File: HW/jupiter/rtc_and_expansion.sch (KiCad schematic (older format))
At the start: 3 parts, among them J2 Expansion Bus, U3 DS1511Y+

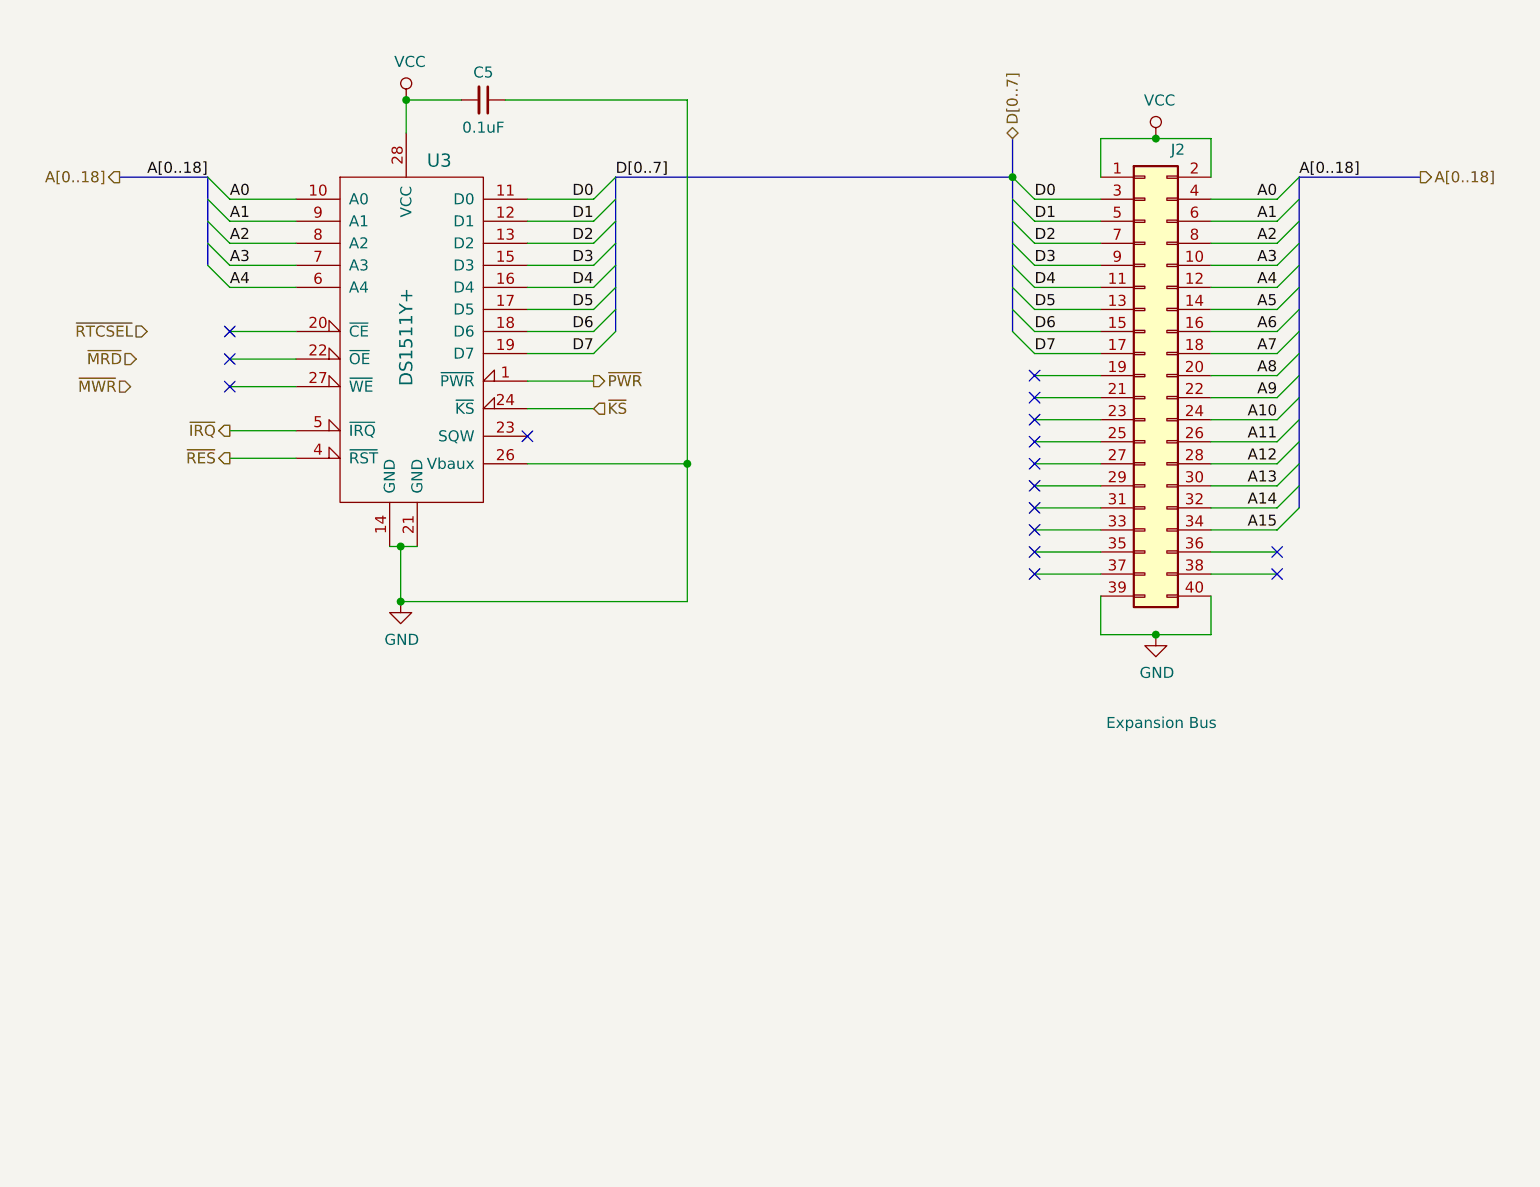
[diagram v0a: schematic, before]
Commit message: A lot of new data sheets. Some updates to schema and PCB layout.
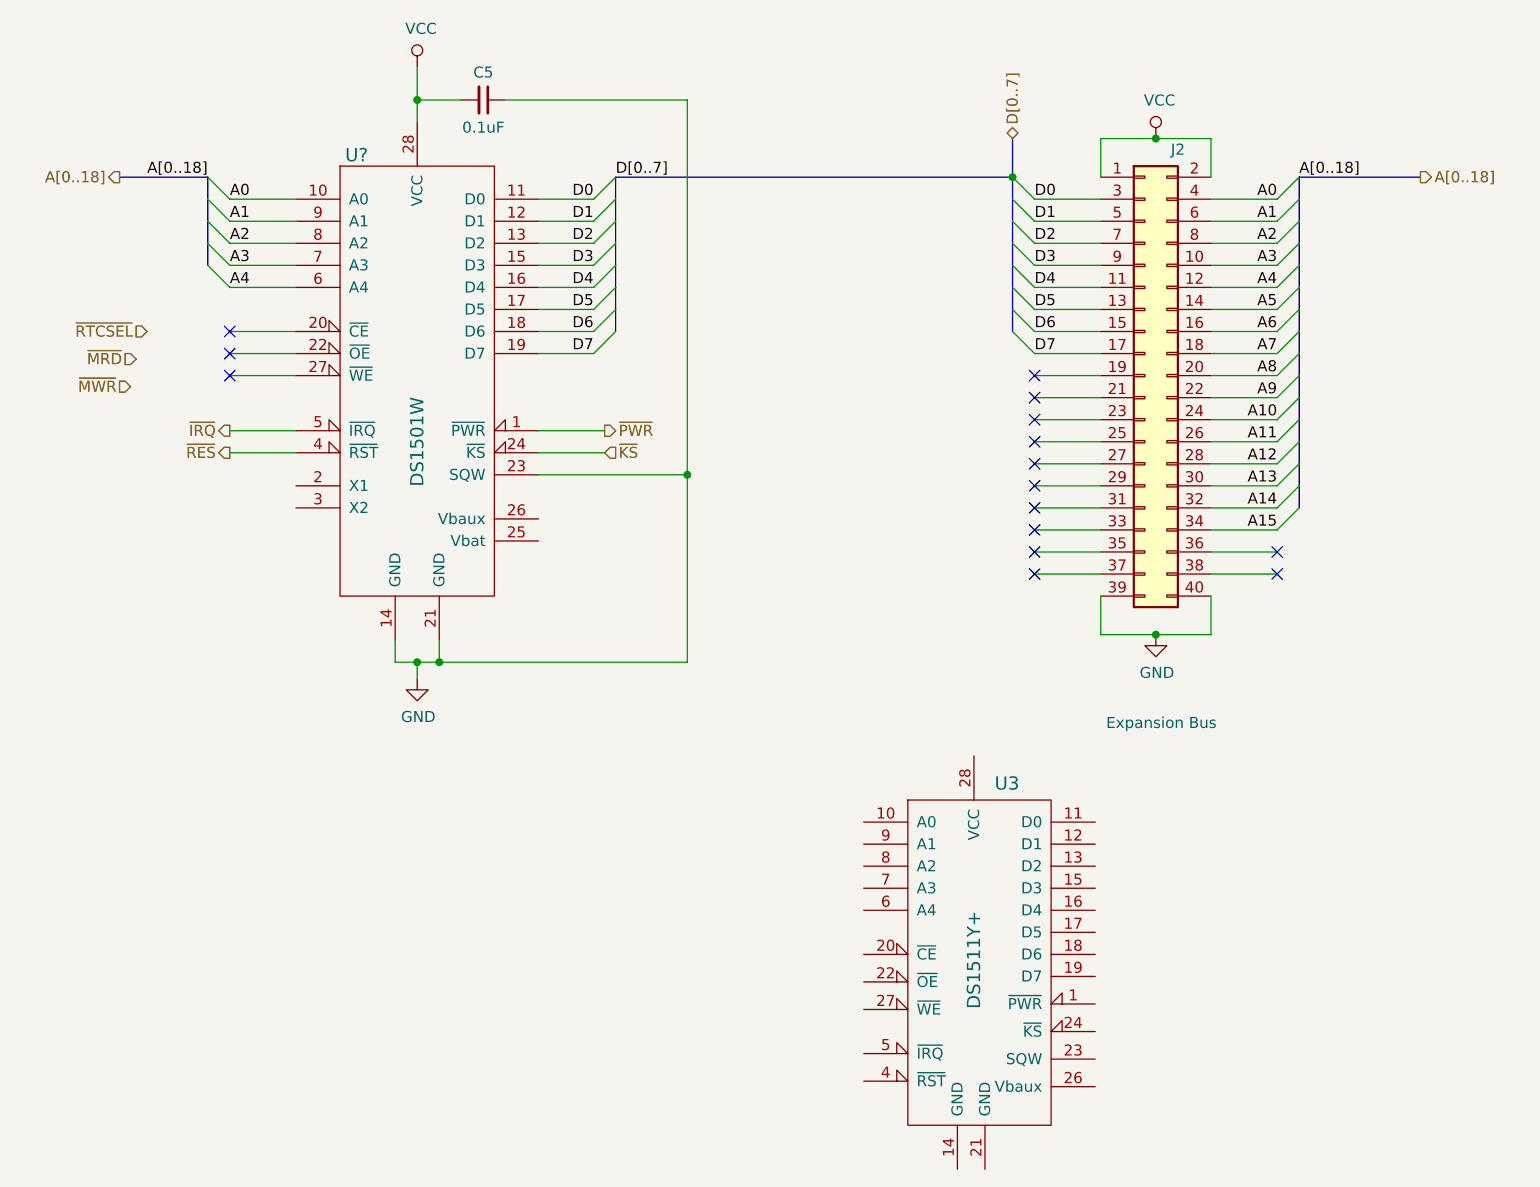
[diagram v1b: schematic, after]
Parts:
- added U?: DS1501W, symbol Grotto:DS1501W
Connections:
- net A0: now also U?.10 (A0); no longer U3.10 (A0)
- net A1: now also U?.9 (A1); no longer U3.9 (A1)
- net A2: now also U?.8 (A2); no longer U3.8 (A2)
- net A3: now also U?.7 (A3); no longer U3.7 (A3)
- net A4: now also U?.6 (A4); no longer U3.6 (A4)
- net D0: now also U?.11 (D0); no longer U3.11 (D0)
- net D1: now also U?.12 (D1); no longer U3.12 (D1)
- net D2: now also U?.13 (D2); no longer U3.13 (D2)
- net D3: now also U?.15 (D3); no longer U3.15 (D3)
- net D4: now also U?.16 (D4); no longer U3.16 (D4)
- net D5: now also U?.17 (D5); no longer U3.17 (D5)
- net D6: now also U?.18 (D6); no longer U3.18 (D6)
- net D7: now also U?.19 (D7); no longer U3.19 (D7)
- net GND: now also U?.14 (GND), U?.21 (GND), U?.23 (SQW); no longer U3.14 (GND), U3.21 (GND), U3.26 (Vbaux)
- net VCC: now also U?.28 (VCC); no longer U3.28 (VCC)
- net ~IRQ: now also U?.5 (~IRQ); no longer U3.5 (~IRQ)
- net ~KS: now also U?.24 (~KS); no longer U3.24 (~KS)
- net ~PWR: now also U?.1 (~PWR); no longer U3.1 (~PWR)
- net ~RES: now also U?.4 (~RST); no longer U3.4 (~RST)
- no-connect marks 16 -> 15
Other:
- moved on the sheet: U3
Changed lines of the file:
@@
 EESchema Schematic File Version 4
 LIBS:jupiter-cache
-EELAYER 29 0
+EELAYER 30 0
 EELAYER END
 $Descr A4 11693 8268
 encoding utf-8
-Sheet 3 4
+Sheet 3 5
 Title ""
 Date ""
@@
 L Grotto:DS1511Y+ U3
 U 1 1 5D100309
-P 2675 2775
-F 0 "U3" H 2850 3525 60  0000 C CNN
-F 1 "DS1511Y+" V 2700 2725 60  0000 C CNN
-F 2 "Package_DIP:DIP-28_W15.24mm_Socket" H 2425 3225 60  0001 C CNN
-F 3 "" H 2425 3225 60  0001 C CNN
-	1    2675 2775
+P 5250 5600
+F 0 "U3" H 5425 6350 60  0000 C CNN
+F 1 "DS1511Y+" V 5275 5550 60  0000 C CNN
+F 2 "Package_DIP:DIP-28_W15.24mm_Socket" H 5000 6050 60  0001 C CNN
+F 3 "" H 5000 6050 60  0001 C CNN
+	1    5250 5600
 	1    0    0    -1
 $EndComp
@@
 D7
 Wire Wire Line
-	3250 2200 3550 2200
-Wire Wire Line
-	3250 2300 3550 2300
-Wire Wire Line
-	3250 2400 3550 2400
-Wire Wire Line
-	3250 2500 3550 2500
-Wire Wire Line
-	3250 2600 3550 2600
-Wire Wire Line
-	3250 2700 3550 2700
-Wire Wire Line
-	3250 2800 3550 2800
-Wire Wire Line
-	3250 2900 3550 2900
-Wire Wire Line
-	3250 3025 3550 3025
-Wire Wire Line
-	3250 3150 3550 3150
+	3300 3250 3600 3250
+Wire Wire Line
+	3300 3350 3600 3350
 Wire Wire Line
 	2200 2200 1900 2200
@@
 	2200 2800 1900 2800
 Wire Wire Line
-	2200 2925 1900 2925
-Wire Wire Line
-	2200 3050 1900 3050
+	2200 2900 1900 2900
+Wire Wire Line
+	2200 3000 1900 3000
 Wire Wire Line
 	2200 3250 1900 3250
 Wire Wire Line
-	2200 3375 1900 3375
+	2200 3350 1900 3350
 Text Label 3550 2200 2    50   ~ 0
 D0
@@
 L power:GND #PWR011
 U 1 1 5D14AF4F
-P 2675 4025
-F 0 "#PWR011" H 2675 3775 50  0001 C CNN
-F 1 "GND" H 2680 3852 50  0000 C CNN
-F 2 "" H 2675 4025 50  0001 C CNN
-F 3 "" H 2675 4025 50  0001 C CNN
-	1    2675 4025
+P 2750 4375
+F 0 "#PWR011" H 2750 4125 50  0001 C CNN
+F 1 "GND" H 2755 4202 50  0000 C CNN
+F 2 "" H 2750 4375 50  0001 C CNN
+F 3 "" H 2750 4375 50  0001 C CNN
+	1    2750 4375
 	1    0    0    -1
 $EndComp
@@
 L power:VCC #PWR012
 U 1 1 5D14B363
-P 2700 1750
-F 0 "#PWR012" H 2700 1600 50  0001 C CNN
-F 1 "VCC" H 2717 1923 50  0000 C CNN
-F 2 "" H 2700 1750 50  0001 C CNN
-F 3 "" H 2700 1750 50  0001 C CNN
-	1    2700 1750
-	1    0    0    -1
-$EndComp
-Wire Wire Line
-	2700 1900 2700 1750
-Wire Wire Line
-	2700 1750 2950 1750
-Connection ~ 2700 1750
+P 2750 1600
+F 0 "#PWR012" H 2750 1450 50  0001 C CNN
+F 1 "VCC" H 2767 1773 50  0000 C CNN
+F 2 "" H 2750 1600 50  0001 C CNN
+F 3 "" H 2750 1600 50  0001 C CNN
+	1    2750 1600
+	1    0    0    -1
+$EndComp
+Wire Wire Line
+	2750 1750 2950 1750
 Wire Wire Line
 	3150 1750 3975 1750
-Wire Wire Line
-	3975 1750 3975 3400
-Wire Wire Line
-	3975 4025 2675 4025
-Wire Wire Line
-	2750 3775 2675 3775
-Wire Wire Line
-	2675 4025 2675 3775
-Connection ~ 2675 4025
-Connection ~ 2675 3775
-Wire Wire Line
-	2675 3775 2625 3775
-Wire Wire Line
-	3250 3400 3975 3400
-Connection ~ 3975 3400
-Wire Wire Line
-	3975 3400 3975 4025
-NoConn ~ 3250 3275
 Wire Bus Line
 	3650 2100 5450 2100
@@
 Text HLabel 1900 3250 0    50   Output ~ 0
 ~IRQ
-Text HLabel 1900 3375 0    50   Output ~ 0
+Text HLabel 1900 3350 0    50   Output ~ 0
 ~RES
-Text HLabel 3550 3025 2    50   Output ~ 0
+Text HLabel 3600 3250 2    50   Output ~ 0
 ~PWR
-Text HLabel 3550 3150 2    50   Input ~ 0
+Text HLabel 3600 3350 2    50   Input ~ 0
 ~KS
 Text HLabel 1450 3050 0    50   Input ~ 0
@@
 NoConn ~ 6650 3900
 NoConn ~ 1900 2800
-NoConn ~ 1900 2925
-NoConn ~ 1900 3050
+NoConn ~ 1900 2900
+NoConn ~ 1900 3000
+Wire Wire Line
+	3300 2200 3550 2200
+Wire Wire Line
+	3300 2300 3550 2300
+Wire Wire Line
+	3300 2400 3550 2400
+Wire Wire Line
+	3300 2500 3550 2500
+Wire Wire Line
+	3300 2600 3550 2600
+Wire Wire Line
+	3300 2700 3550 2700
+Wire Wire Line
+	3300 2800 3550 2800
+Wire Wire Line
+	3300 2900 3550 2900
+Wire Wire Line
+	3975 1750 3975 3450
+Wire Wire Line
+	3300 3450 3975 3450
+Wire Wire Line
+	2750 1600 2750 1750
+Wire Wire Line
+	2750 1750 2750 1850
+Connection ~ 2750 1750
+$Comp
+L Grotto:DS1501W U?
+U 1 1 5DA42BF4
+P 2750 2750
+F 0 "U?" H 2475 3500 60  0000 C CNN
+F 1 "DS1501W" V 2750 2200 60  0000 C CNN
+F 2 "" H 2450 3200 60  0001 C CNN
+F 3 "" H 2450 3200 60  0001 C CNN
+	1    2750 2750
+	1    0    0    -1
+$EndComp
+Connection ~ 3975 3450
+Wire Wire Line
+	2650 4200 2650 4300
+Wire Wire Line
+	2650 4300 2750 4300
+Wire Wire Line
+	2850 4300 2850 4200
+Wire Wire Line
+	2750 4300 2750 4375
+Connection ~ 2750 4300
+Wire Wire Line
+	2750 4300 2850 4300
+Wire Wire Line
+	3975 4300 2850 4300
+Wire Wire Line
+	3975 3450 3975 4300
+Connection ~ 2850 4300
 Wire Bus Line
 	1800 2100 1800 2500
